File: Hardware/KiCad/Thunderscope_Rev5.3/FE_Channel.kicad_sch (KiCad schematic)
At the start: 105 parts, among them J1002_4 BNC, J3_4 UFL, J4_4 UFL, K1000_4 UD2-4.5NUN-L, K1001_4 UD2-4.5NUN-L, Q1002_4 DMN62D0UW, Q1003_4 DMN62D0UW, U1001_4 TMUX4053, U1008_4 LMH6518, U1009_4 BUF802, U1011_4 OPA140AIDBVR

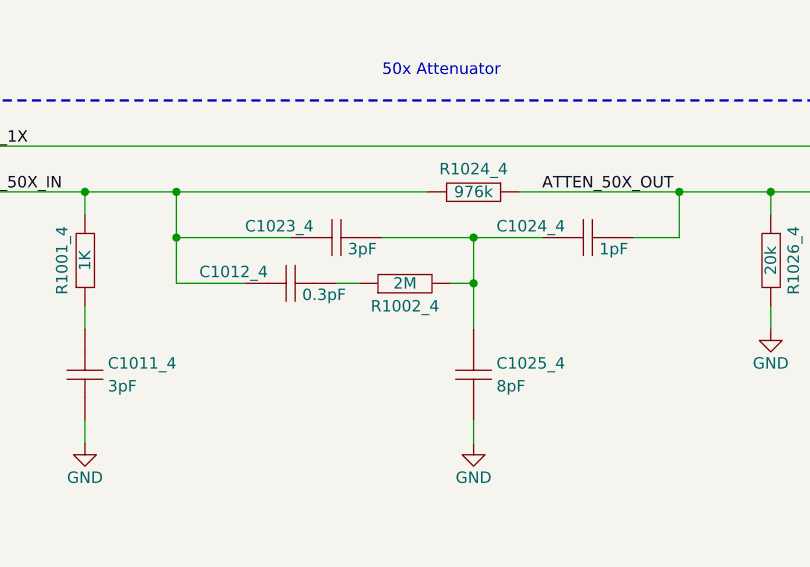
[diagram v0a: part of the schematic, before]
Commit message: Changed R1002 to 976k as per #408
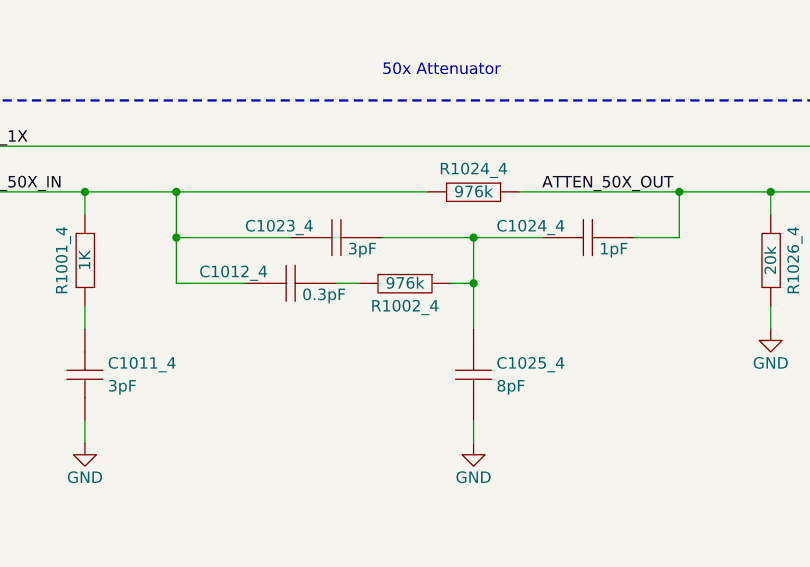
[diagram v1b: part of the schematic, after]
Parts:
- R1002_4: value 2M -> 976k; symbol Thunderscope_Rev5:RES 2M OHM 1% 1/10W 0402 -> Thunderscope_Rev5:RES 976k OHM 1% 1/10W 0402; MANUFACTURER PART NUMBER RK73H1ETTP2004F -> RK73H1ETTP9763F; SUPPLIER PART NUMBER 1 660-RK73H1ETTP2004F -> 660-RK73H1ETTP9763F
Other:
- moved on the sheet: R1002_4
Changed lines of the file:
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@@
 	)
 	(symbol
-		(lib_id "Thunderscope_Rev5:RES 2M OHM 1% 1/10W 0402")
-		(at 269.24 48.26 180)
+		(lib_id "Thunderscope_Rev5:RES 976k OHM 1% 1/10W 0402")
+		(at 269.24 48.26 0)
 		(unit 1)
 		(exclude_from_sim no)
@@
 			)
 		)
-		(property "Value" "2M"
+		(property "Value" "976k"
 			(at 269.24 48.26 0)
 			(effects
@@
 			)
 		)
-		(property "SUPPLIER PART NUMBER 1" "660-RK73H1ETTP2004F"
+		(property "SUPPLIER PART NUMBER 1" "660-RK73H1ETTP9763F"
 			(at 269.24 48.26 0)
 			(effects
@@
 			)
 		)
-		(property "MANUFACTURER PART NUMBER" "RK73H1ETTP2004F"
+		(property "MANUFACTURER PART NUMBER" "RK73H1ETTP9763F"
 			(at 269.24 48.26 0)
 			(effects
